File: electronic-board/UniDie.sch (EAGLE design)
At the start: 24 parts, among them IC1 ATMEGA88-THIN, J2 AVR_SPI_PROG_3X2NS

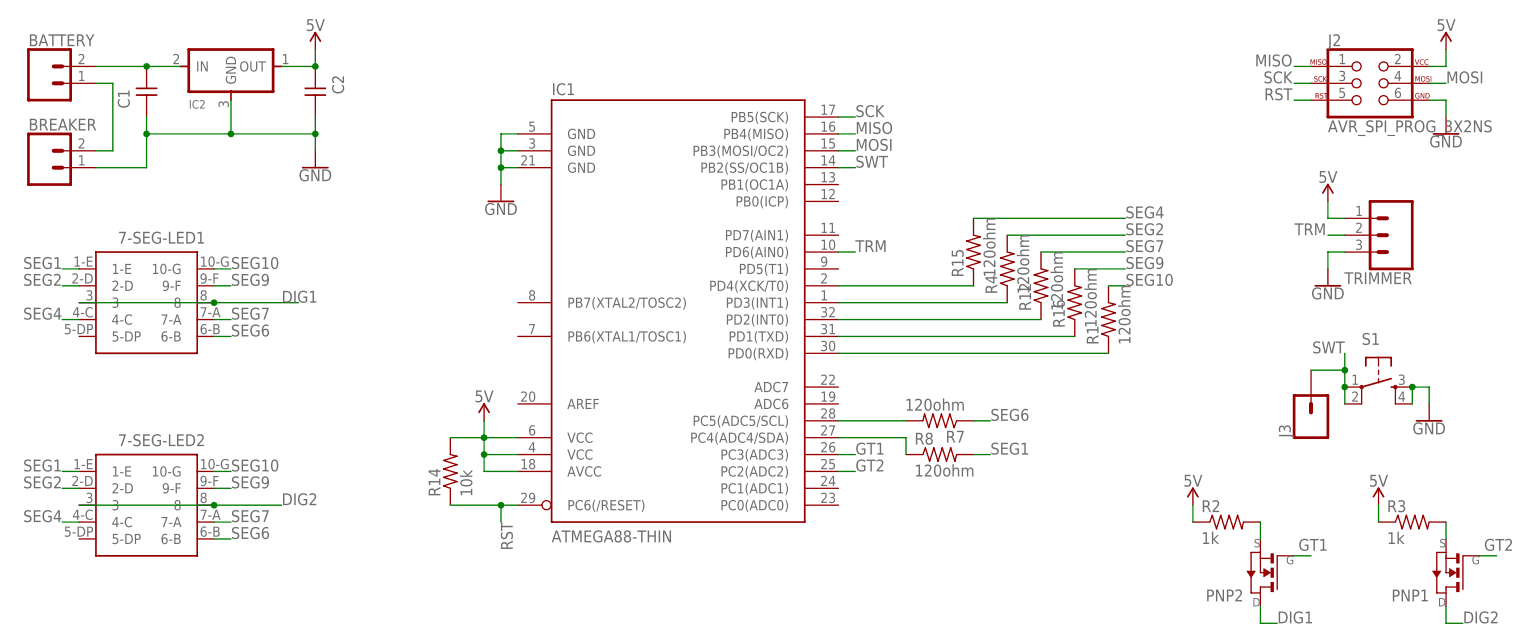
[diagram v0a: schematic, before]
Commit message: Adapted parts and routes for milling. Prepared milling files
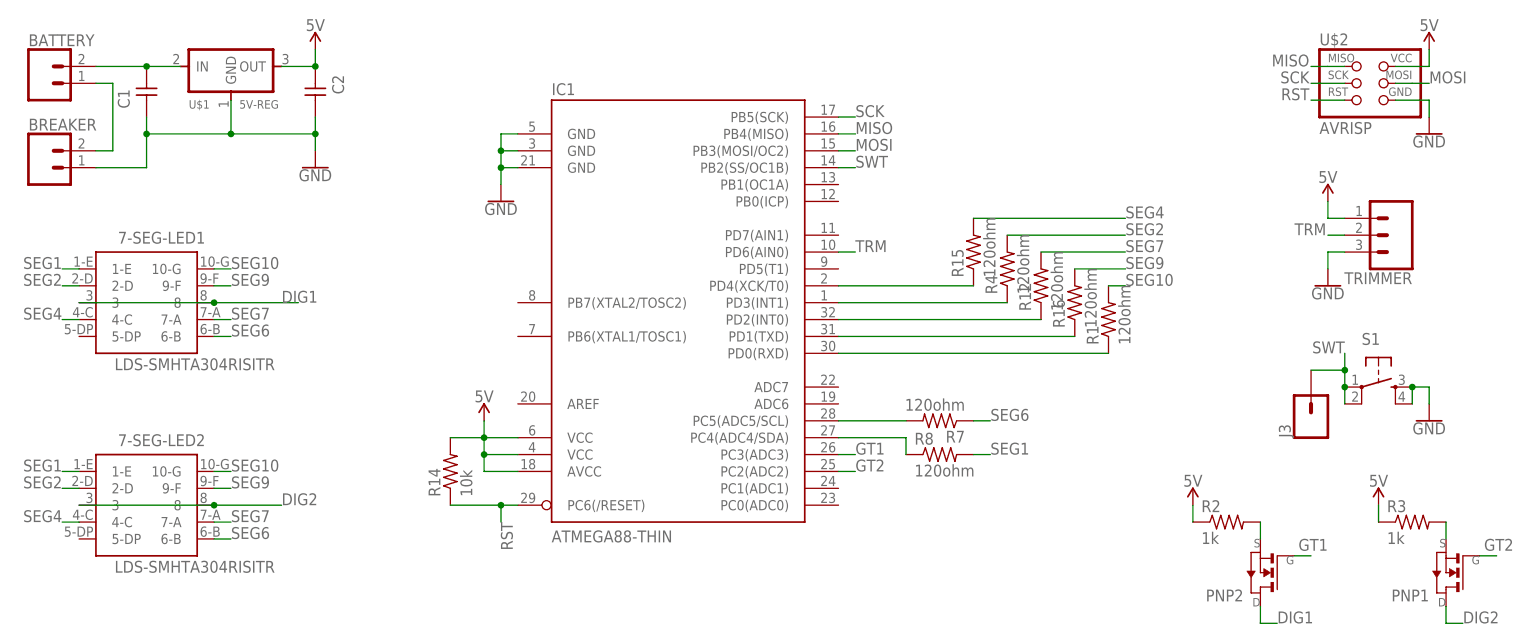
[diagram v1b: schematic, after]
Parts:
- removed IC2: (no value), fab:REGULATORSOT23
- removed J2: AVR_SPI_PROG_3X2NS, SparkFun-Connectors:AVR_SPI_PROG_3X2NS
- added U$1: 5V-REG, AG:5V-REG
- added U$2: AVRISP, fab:AVRISP
- 7-SEG-LED1, 7-SEG-LED2: value (none) -> LDS-SMHTA304RISITR
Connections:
- net 5V: now also U$1.OUT, U$2.VCC; no longer IC2.OUT, J2.2
- net GND: now also U$1.GND, U$2.GND; no longer IC2.GND, J2.6
- net MISO: now also U$2.MISO; no longer J2.1
- net MOSI: now also U$2.MOSI; no longer J2.4
- net N$1: now also U$1.IN; no longer IC2.IN
- net RST: now also U$2.RST; no longer J2.5
- net SCK: now also U$2.SCK; no longer J2.3

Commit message: Revert "Adapted parts and routes for milling. Prepared milling files"
This reverts commit d229ee454f50b57581f4fd08392e80f763665f52.
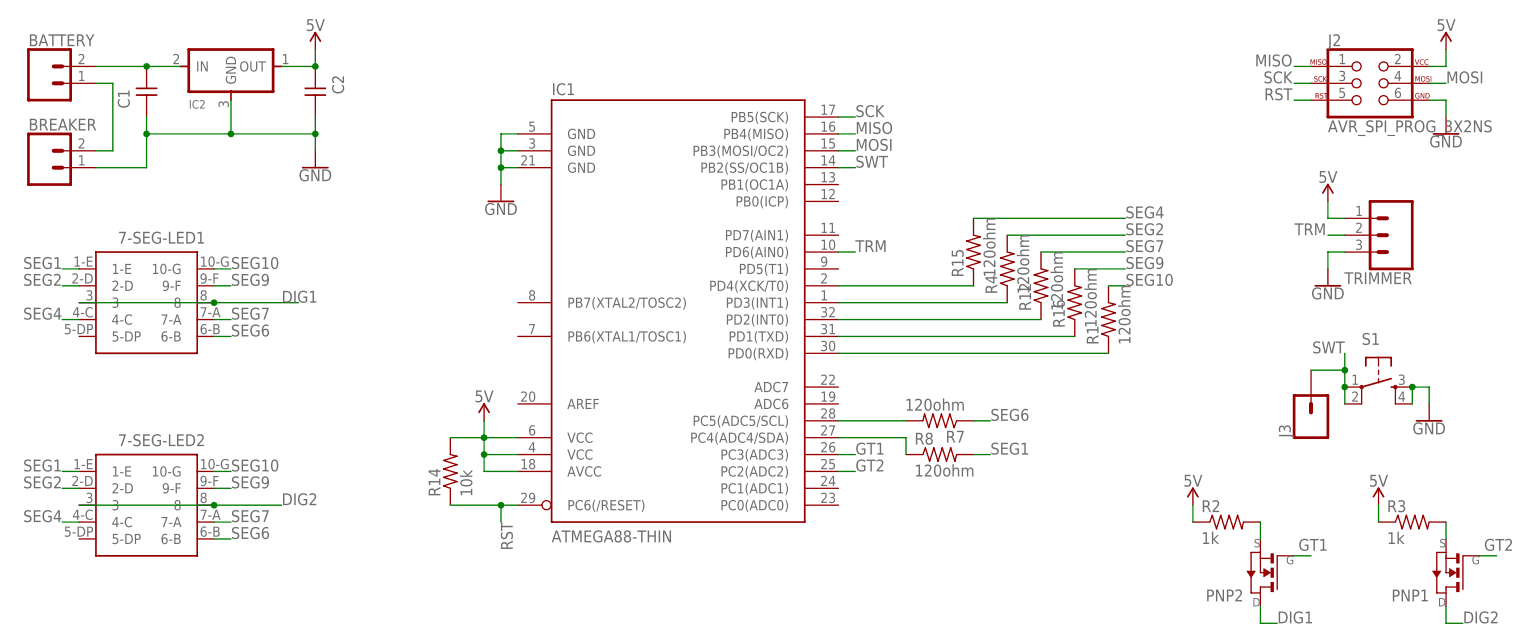
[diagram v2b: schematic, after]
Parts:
- removed U$1: 5V-REG, AG:5V-REG
- removed U$2: AVRISP, fab:AVRISP
- added IC2: (no value), fab:REGULATORSOT23
- added J2: AVR_SPI_PROG_3X2NS, SparkFun-Connectors:AVR_SPI_PROG_3X2NS
- 7-SEG-LED1, 7-SEG-LED2: value LDS-SMHTA304RISITR -> (none)
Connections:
- net 5V: now also IC2.OUT, J2.2; no longer U$1.OUT, U$2.VCC
- net GND: now also IC2.GND, J2.6; no longer U$1.GND, U$2.GND
- net MISO: now also J2.1; no longer U$2.MISO
- net MOSI: now also J2.4; no longer U$2.MOSI
- net N$1: now also IC2.IN; no longer U$1.IN
- net RST: now also J2.5; no longer U$2.RST
- net SCK: now also J2.3; no longer U$2.SCK
